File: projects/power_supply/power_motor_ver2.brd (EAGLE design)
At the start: 120 x 59 mm, 18 parts

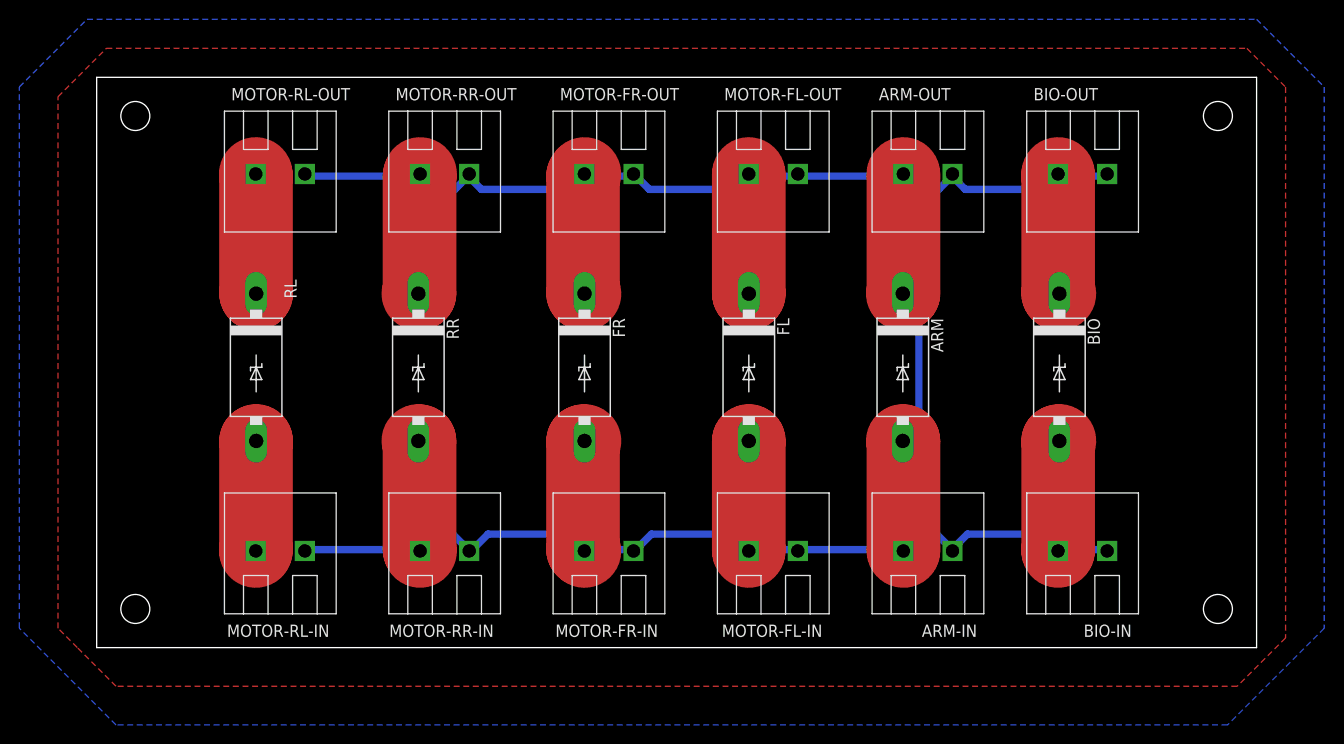
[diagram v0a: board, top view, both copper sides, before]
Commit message: aa
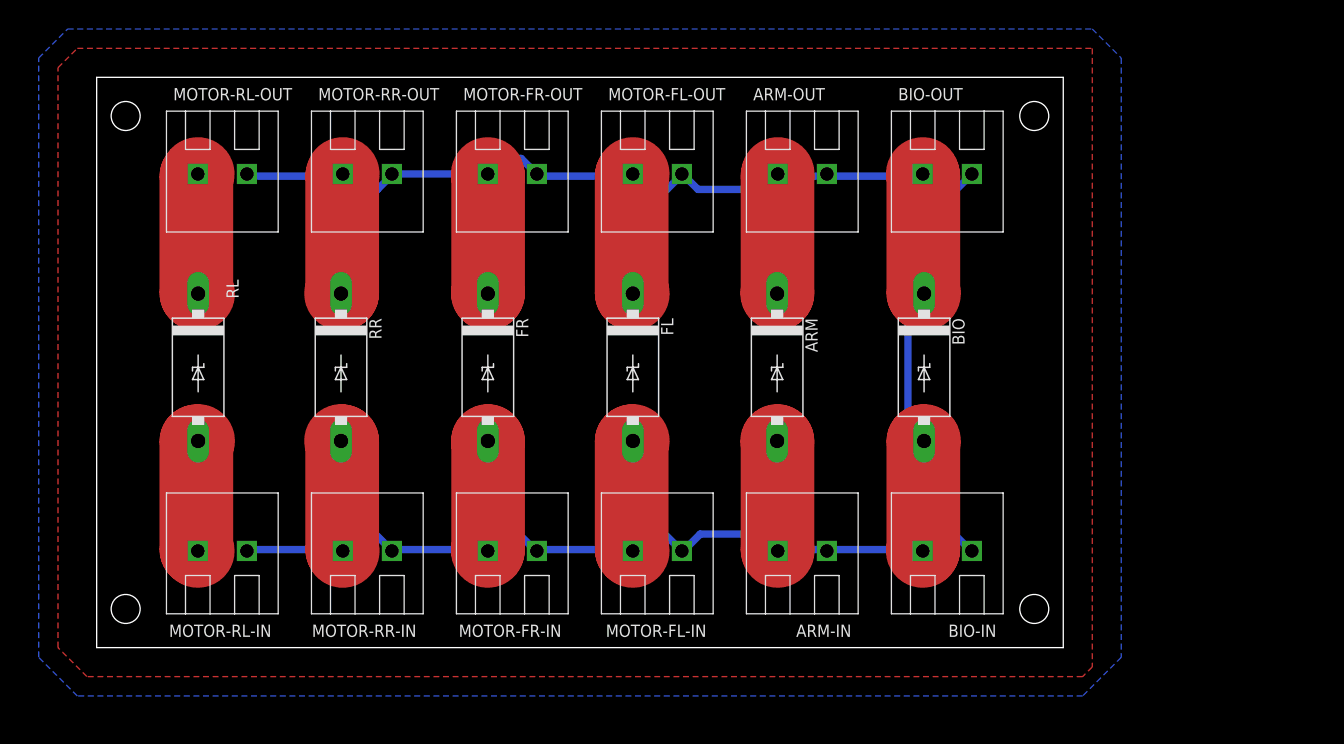
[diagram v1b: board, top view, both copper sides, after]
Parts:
- moved BIO 14.0 mm to (82.6, 20.0)
- moved BIO-IN 14.0 mm to (85.0, 1.00)
- moved BIO-OUT 14.0 mm to (85.0, 40.0)
- moved ARM 13.0 mm to (67.4, 20.0)
- moved ARM-IN 13.0 mm to (70.0, 1.00)
- moved ARM-OUT 13.0 mm to (70.0, 40.0)
- moved FL 12.0 mm to (52.5, 20.0)
- moved MOTOR-FL-IN 12.0 mm to (55.0, 1.00)
- moved MOTOR-FL-OUT 12.0 mm to (55.0, 40.0)
- moved FR 10.0 mm to (37.5, 20.0)
- moved MOTOR-FR-IN 10.0 mm to (40.0, 1.00)
- moved MOTOR-FR-OUT 10.0 mm to (40.0, 40.0)
- moved MOTOR-RR-IN 8.00 mm to (25.0, 1.00)
- moved MOTOR-RR-OUT 8.00 mm to (25.0, 40.0)
- moved RR 8.00 mm to (22.3, 20.0)
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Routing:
- net GND: track 216.1 -> 199.8 mm
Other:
- board size 120 x 59 mm -> 100 x 59 mm
